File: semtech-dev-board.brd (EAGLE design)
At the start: 73.4 x 100 mm, 58 parts, among them Q1 BSS123, U1 SEMTECH_SX1236, U3 MIC5219 3.3V, X1 BU-SMA-G, X2 BU-SMA-G, X3 BU-SMA-G, X4 BU-SMA-G

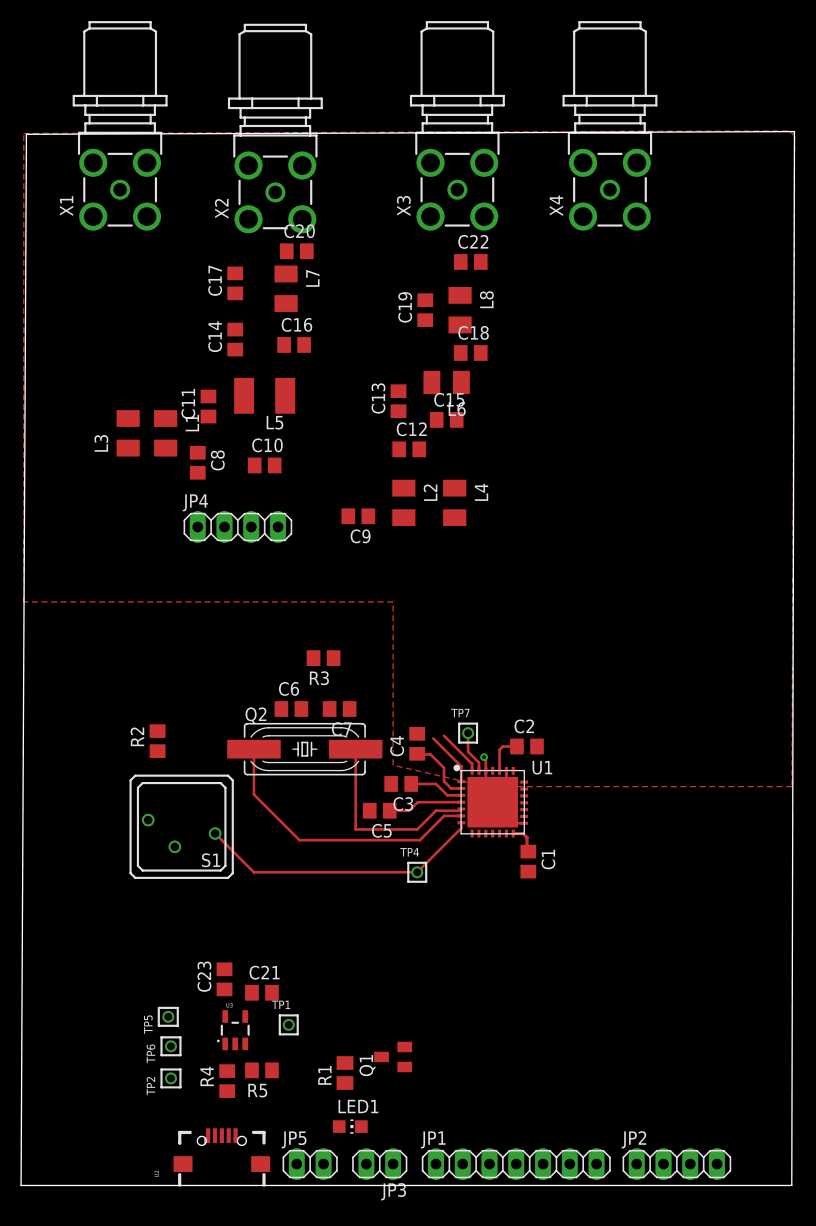
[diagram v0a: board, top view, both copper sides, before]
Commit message: board draft
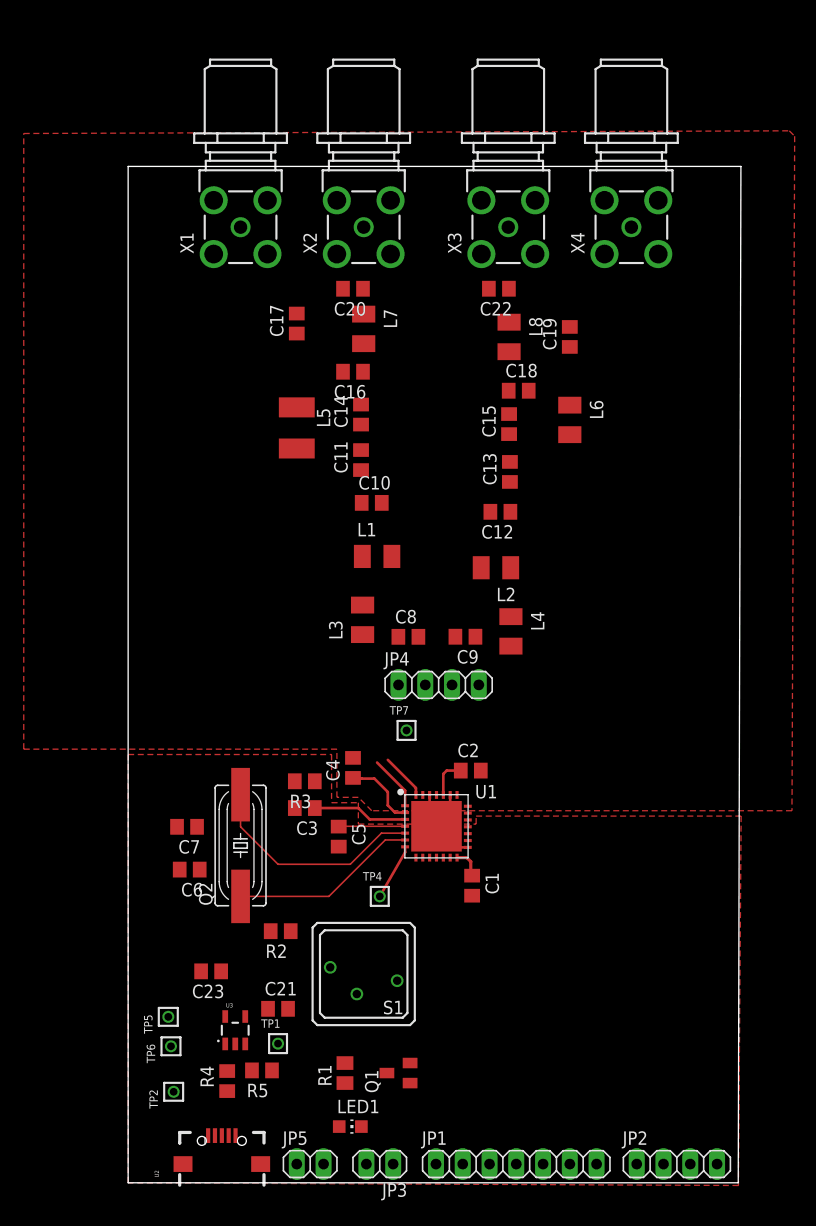
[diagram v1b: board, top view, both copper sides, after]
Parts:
- moved L3 28.4 mm to (39.3, 53.7)
- moved C8 25.9 mm to (43.6, 52.1), turned to 0 degrees
- moved JP4 24.2 mm to (46.5, 47.5)
- moved L1 23.2 mm to (40.6, 59.7), turned to 0 degrees
- moved S1 22.2 mm to (39.4, 20.1)
- moved R2 21.5 mm to (31.5, 24.1), turned to 180 degrees
- moved C7 18.3 mm to (22.6, 34.0)
- moved C6 18.0 mm to (22.9, 30.0), turned to 180 degrees
- moved C11 15.3 mm to (39.1, 68.8)
- moved C9 15.3 mm to (49.0, 52.1)
- moved C19 13.9 mm to (58.9, 80.5)
- moved C14 13.9 mm to (39.1, 73.2)
- moved L4 13.3 mm to (53.3, 52.6)
- moved C13 12.5 mm to (53.2, 67.7)
- moved L6 12.2 mm to (58.9, 72.6), turned to 270 degrees
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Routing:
- net SX1236_RST: track 27.1 -> 5.34 mm
- net XTALB: track 26.7 -> 17.8 mm
- net N$2: track 18.4 -> 22.9 mm
- net PA_BOOST: track 4.01 -> 0.00 mm
- net VBAT: track 11.8 -> 15.6 mm
- net GND: track 12.0 -> 10.6 mm, vias 1 -> 0
- net VR_DIG: track 7.13 -> 6.32 mm
- net VR_ANA: track 6.29 -> 7.03 mm
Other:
- board size 73.4 x 100 mm -> 58.1 x 96.4 mm
